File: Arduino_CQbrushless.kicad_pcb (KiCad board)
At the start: 2 copper layers, 70.4 x 81.8 mm, 3 parts, among them J1 Nucleo_F302R8, J2 AE-LLCNV8-DIP20

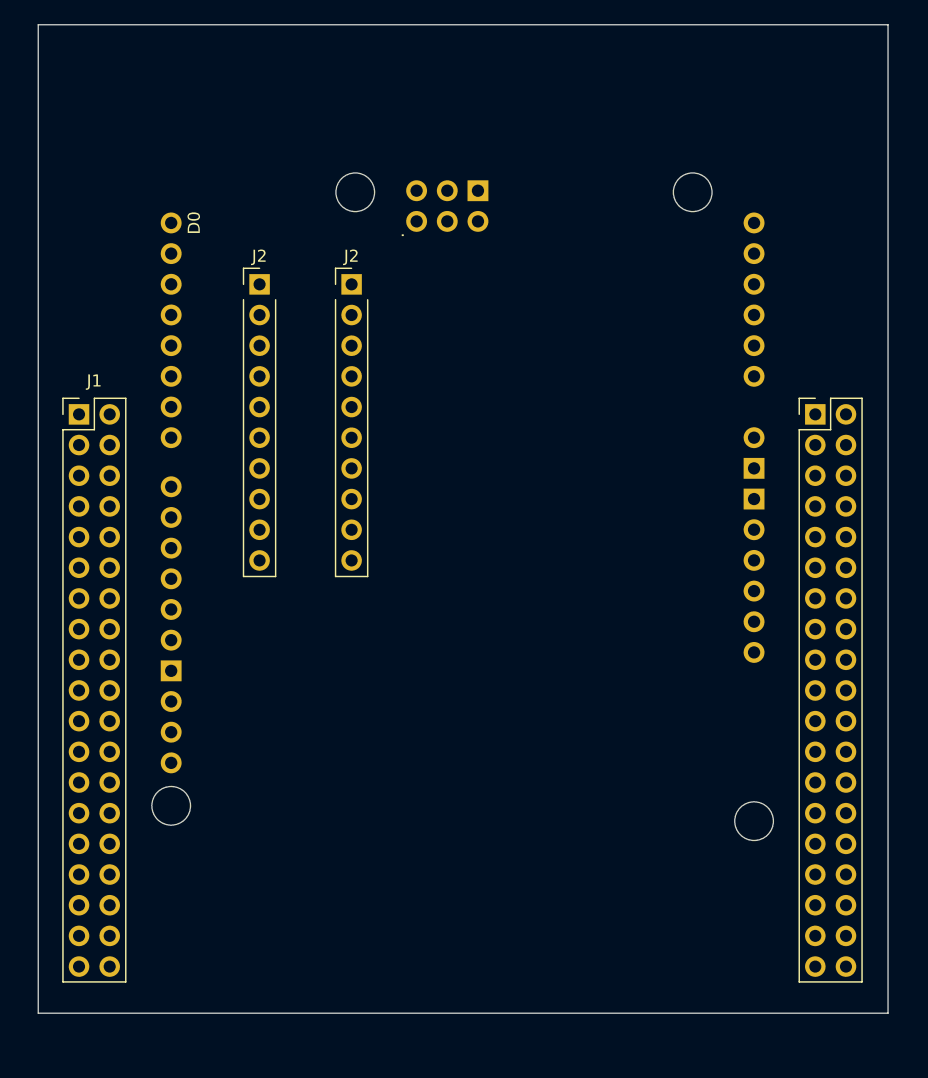
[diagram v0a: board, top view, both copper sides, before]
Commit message: 1228
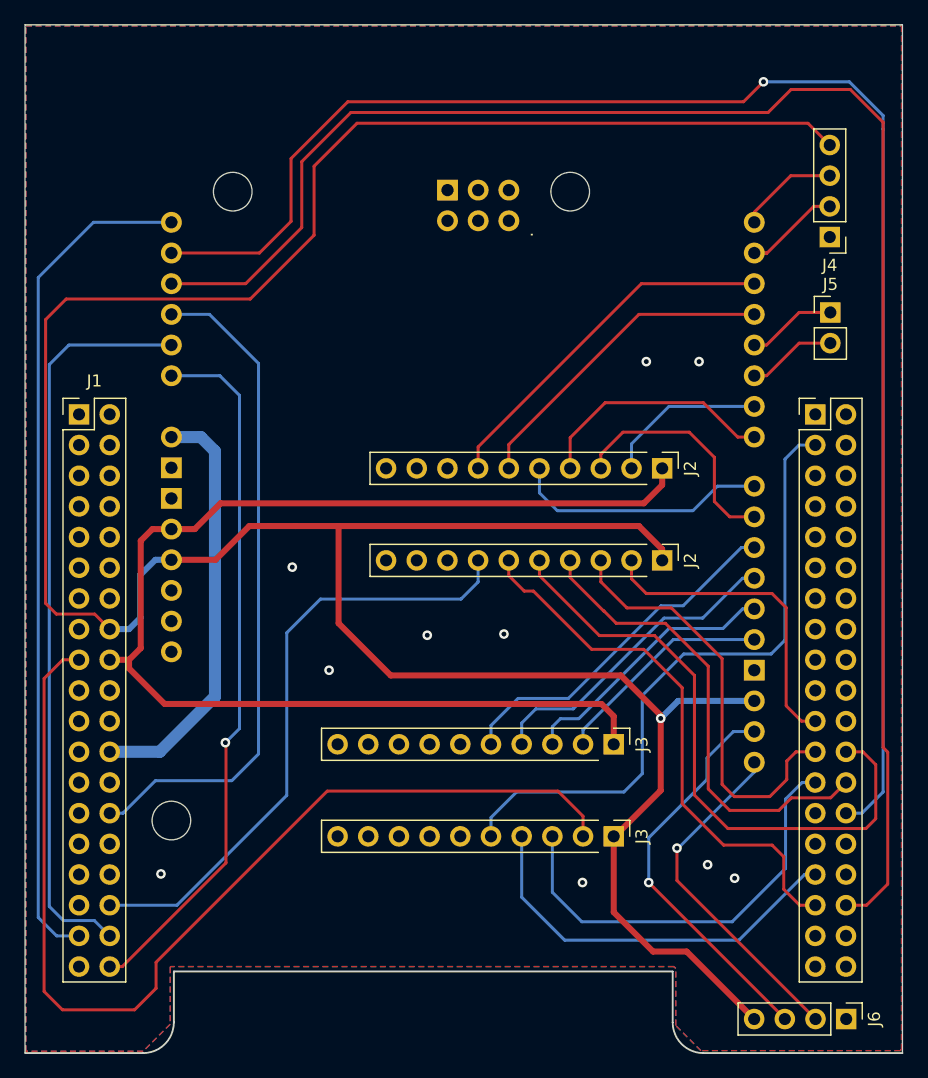
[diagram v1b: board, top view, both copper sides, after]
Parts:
- added J3: AE-LLCNV8-DIP20, Library:AE-LLCNV8-DIP, F.Cu at (129.1, 137.4)
- added J4: Conn_01x04, Connector_PinHeader_2.54mm:PinHeader_1x04_P2.54mm_Vertical, F.Cu at (147.0, 95.4)
- added J5: Conn_01x02, Connector_PinHeader_2.54mm:PinHeader_1x02_P2.54mm_Vertical, F.Cu at (147.0, 101.6)
- added J6: Conn_01x04, Connector_PinHeader_2.54mm:PinHeader_1x04_P2.54mm_Vertical, F.Cu at (148.3, 160.1)
- moved J2 36.7 mm to (133.1, 114.6), turned to -90 degrees
- moved A1 0.53 mm to (143.8, 157.7)
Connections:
- A1 pad 3V3: /+3.3V -> +3.3V
- A1 pad 5V1: /+5V -> +5V
- A1 pad AREF: /+3.3V -> +3.3V
- A1 pad D0: unconnected-(A1-D0/RX-PadD0) -> Net-(A1-D0/RX)
- A1 pad D1: unconnected-(A1-D1/TX-PadD1) -> Net-(A1-D1/TX)
- A1 pad D10: Net-(J2-A7) -> Net-(J3-A3)
- A1 pad D11: Net-(J2-GND) -> Net-(J3-A2)
- A1 pad D12: unconnected-(A1-PadD12) -> Net-(J3-A1)
- A1 pad D13: unconnected-(A1-PadD13) -> Net-(J3-A0)
- A1 pad D2: Net-(J2-VA) -> Net-(J2-A5)
- A1 pad D3: Net-(J2-A0) -> Net-(J2-A4)
- A1 pad D4: Net-(J2-A1) -> Net-(J5-Pin_1)
- A1 pad D5: Net-(J2-A2) -> Net-(J5-Pin_2)
- A1 pad D6: Net-(J2-A3) -> Net-(J2-A0)
- A1 pad D7: Net-(J2-A4) -> Net-(J2-A2)
- A1 pad D8: Net-(J2-A5) -> Net-(J2-A3)
- A1 pad D9: Net-(J2-A6) -> Net-(J2-A1)
- A1 pad SCL: unconnected-(A1-PadSCL) -> Net-(J6-Pin_2)
- A1 pad SDA: unconnected-(A1-PadSDA) -> Net-(J6-Pin_3)
- J1 pad 16: /+3.3V -> +3.3V
- J1 pad 18: /+5V -> +5V
- J2 pad 1: Net-(J2-VA) -> +5V
- J2 pad 10: Net-(J2-GND) -> GND
- J2 pad 11: /T_HIN -> GND
- J2 pad 12: /_R_LIN -> unconnected-(J2-B7-Pad12)
- J2 pad 13: /R_HIN -> unconnected-(J2-B6-Pad13)
- J2 pad 14: /_T_LIN -> /_S_LIN
- J2 pad 15: /S_HIN -> /T_HIN
- J2 pad 16: /_S_LIN -> /_T_LIN
- J2 pad 17: /Direction -> /_R_LIN
- J2 pad 18: /HV -> /R_HIN
- J2 pad 19: /HW -> /S_HIN
- J2 pad 20: /HU -> +3.3V
- J2 pad 8: Net-(J2-A6) -> unconnected-(J2-A6-Pad8)
- J2 pad 9: Net-(J2-A7) -> unconnected-(J2-A7-Pad9)
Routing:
- net +3.3V: track 0.00 -> 238.0 mm, vias 0 -> 1
- net Net-(A1-PadA3): track 0.00 -> 137.3 mm
- net Net-(A1-PadA4): track 0.00 -> 128.9 mm, vias 0 -> 1
- net +5V: track 0.00 -> 103.1 mm
- net /HU: track 0.00 -> 86.0 mm
- net /ACCEL: track 0.00 -> 69.9 mm
- net /S_sense: track 0.00 -> 61.7 mm
- net /T_sense: track 0.00 -> 58.7 mm, vias 0 -> 1
- net /R_sense: track 0.00 -> 55.6 mm
- net /Direction: track 0.00 -> 53.8 mm
- net /_T_LIN: track 0.00 -> 51.3 mm
- net /_S_LIN: track 0.00 -> 51.3 mm
- net /T_HIN: track 0.00 -> 45.1 mm
- net /_R_LIN: track 0.00 -> 39.2 mm
- net /HW: track 0.00 -> 35.6 mm
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- added copper zone on B.Cu, net GND
- added copper zone on F.Cu, net GND
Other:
- board size 70.4 x 81.8 mm -> 72.6 x 85.1 mm
